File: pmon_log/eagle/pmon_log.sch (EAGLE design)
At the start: 29 parts, among them J5 microSD Socket, Q1 16Mhz, U2 LTC2943, U3 TC1015, U4 ATMEGA328TQFP32

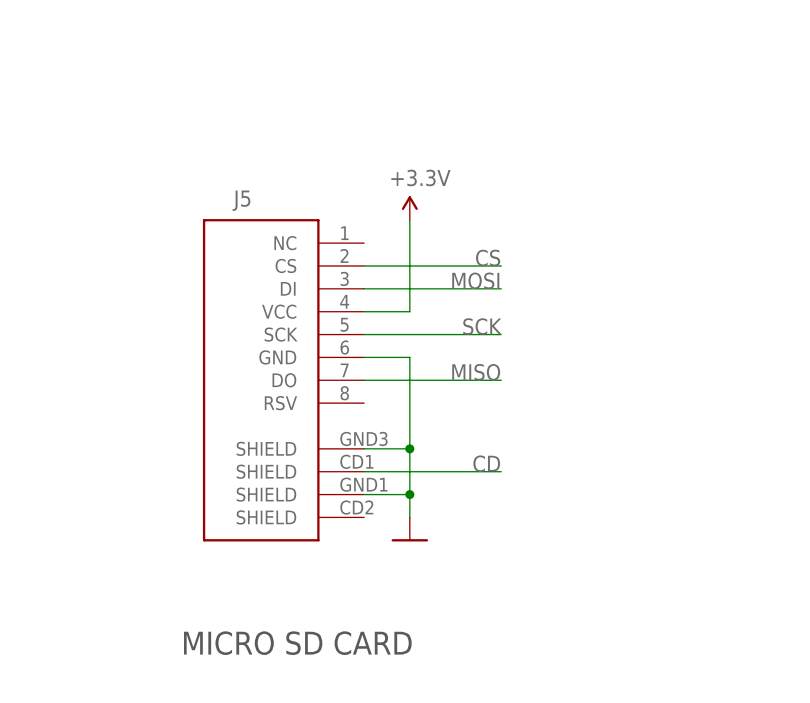
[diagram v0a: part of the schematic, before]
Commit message: Added pdf schematic.
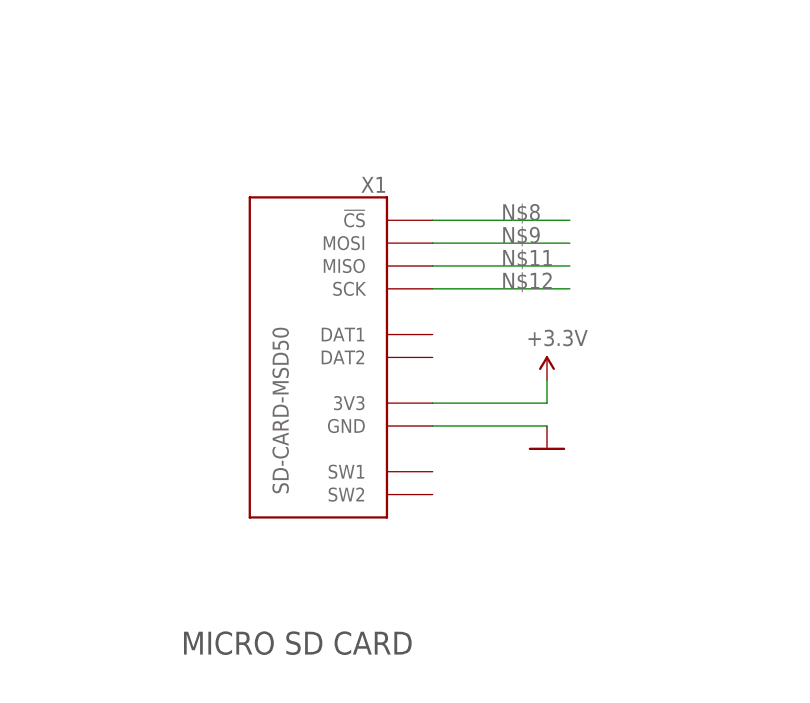
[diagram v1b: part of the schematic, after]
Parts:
- removed J5: microSD Socket, SparkFun:USD-SOCKETNEW
- added X1: SD-CARD-MSD50, pmon_log:SD-CARD-MSD50
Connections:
- new net N$11: X1.MISO
- new net N$12: X1.SCK
- new net N$8: X1.!CS
- new net N$9: X1.MOSI
- net +3.3V: now also X1.3V3; no longer J5.VCC
- net CD: no longer J5.SHIELD@2
- net CS: no longer J5.CS
- net GND: now also X1.GND; no longer J5.GND, J5.SHIELD@1, J5.SHIELD@3
- net MISO: no longer J5.DO
- net MOSI: no longer J5.DI
- net SCK: no longer J5.SCK
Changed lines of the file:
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@@
 <layer number="108" name="tplace-old" color="7" fill="1" visible="yes" active="yes"/>
 <layer number="109" name="ref-old" color="7" fill="1" visible="yes" active="yes"/>
+<layer number="110" name="fp0" color="7" fill="1" visible="yes" active="yes"/>
 <layer number="116" name="Patch_BOT" color="9" fill="4" visible="yes" active="yes"/>
 <layer number="118" name="Rect_Pads" color="7" fill="1" visible="yes" active="yes"/>
+<layer number="120" name="Descript" color="7" fill="1" visible="yes" active="yes"/>
 <layer number="121" name="_tsilk" color="7" fill="1" visible="yes" active="yes"/>
 <layer number="122" name="_bsilk" color="7" fill="1" visible="yes" active="yes"/>
+<layer number="123" name="tTestmark" color="7" fill="1" visible="yes" active="yes"/>
+<layer number="124" name="bTestmark" color="7" fill="1" visible="yes" active="yes"/>
 <layer number="125" name="_tNames" color="7" fill="1" visible="no" active="yes"/>
 <layer number="131" name="prix" color="7" fill="1" visible="yes" active="yes"/>
@@
 <part name="J1" library="pmon_log" deviceset="PINHD-1X2" device=""/>
 <part name="J2" library="pmon_log" deviceset="PINHD-1X2" device=""/>
-<part name="J5" library="SparkFun" deviceset="USD-SOCKET" device="NEW" value="microSD Socket"/>
 <part name="U$7" library="pmon_5v" deviceset="NC" device=""/>
 <part name="U$2" library="pmon_log" deviceset="+VBAT" device=""/>
@@
 <part name="D1" library="diode" deviceset="DIODE-" device="SC79_INFINEON"/>
 <part name="U$3" library="pmon_log" deviceset="+VBAT" device=""/>
-<part name="GND2" library="pmon_5v" deviceset="GND" device=""/>
-<part name="U$4" library="pmon_log" deviceset="+3.3V" device=""/>
 <part name="U$9" library="pmon_log" deviceset="+VUSB" device=""/>
 <part name="U$19" library="pmon_log" deviceset="+VUSB" device=""/>
@@
 <part name="R7" library="resistor" deviceset="R-EU_" device="R0402" value="3K3"/>
 <part name="U$6" library="pmon_5v" deviceset="NC" device=""/>
+<part name="X1" library="pmon_log" deviceset="SD-CARD" device="-MSD50"/>
+<part name="U$16" library="pmon_log" deviceset="+3.3V" device=""/>
+<part name="GND9" library="pmon_5v" deviceset="GND" device=""/>
 </parts>
 <sheets>
@@
 <attribute name="VALUE" x="44.45" y="187.96" size="1.778" layer="96"/>
 </instance>
-<instance part="J5" gate="G$1" x="17.78" y="63.5" smashed="yes" rot="MR0">
-<attribute name="NAME" x="12.954" y="80.264" size="1.778" layer="95" rot="MR0"/>
-</instance>
 <instance part="U$7" gate="G$1" x="238.76" y="172.72" rot="R180"/>
 <instance part="U$2" gate="G$1" x="7.62" y="213.36" rot="R270"/>
@@
 <instance part="U$3" gate="G$1" x="91.44" y="215.9" smashed="yes">
 <attribute name="VALUE" x="89.408" y="213.868" size="1.778" layer="96" rot="R90"/>
-</instance>
-<instance part="GND2" gate="1" x="30.48" y="43.18"/>
-<instance part="U$4" gate="G$1" x="30.48" y="78.74" smashed="yes">
-<attribute name="VALUE" x="28.194" y="82.55" size="1.778" layer="96"/>
 </instance>
 <instance part="U$9" gate="G$1" x="121.92" y="121.92" smashed="yes" rot="R270">
@@
 </instance>
 <instance part="U$6" gate="G$1" x="238.76" y="180.34" rot="R180"/>
+<instance part="X1" gate="&gt;NAME" x="20.32" y="63.5" rot="MR0"/>
+<instance part="U$16" gate="G$1" x="45.72" y="60.96" smashed="yes">
+<attribute name="VALUE" x="43.434" y="64.77" size="1.778" layer="96"/>
+</instance>
+<instance part="GND9" gate="1" x="45.72" y="53.34"/>
 </instances>
 <busses>
@@
 </segment>
 <segment>
-<wire x1="25.4" y1="63.5" x2="30.48" y2="63.5" width="0.1524" layer="91"/>
-<wire x1="30.48" y1="63.5" x2="30.48" y2="53.34" width="0.1524" layer="91"/>
-<wire x1="30.48" y1="53.34" x2="30.48" y2="48.26" width="0.1524" layer="91"/>
-<wire x1="30.48" y1="48.26" x2="30.48" y2="45.72" width="0.1524" layer="91"/>
-<wire x1="25.4" y1="53.34" x2="30.48" y2="53.34" width="0.1524" layer="91"/>
-<wire x1="25.4" y1="48.26" x2="30.48" y2="48.26" width="0.1524" layer="91"/>
-<junction x="30.48" y="53.34"/>
-<junction x="30.48" y="48.26"/>
-<pinref part="J5" gate="G$1" pin="GND"/>
-<pinref part="J5" gate="G$1" pin="SHIELD@1"/>
-<pinref part="J5" gate="G$1" pin="SHIELD@3"/>
-<pinref part="GND2" gate="1" pin="GND"/>
-</segment>
-<segment>
 <pinref part="LED1" gate="G$1" pin="C"/>
 <pinref part="GND6" gate="1" pin="GND"/>
@@
 <pinref part="GND7" gate="1" pin="GND"/>
 <wire x1="114.3" y1="55.88" x2="114.3" y2="58.42" width="0.1524" layer="91"/>
+</segment>
+<segment>
+<pinref part="X1" gate="&gt;NAME" pin="GND"/>
+<wire x1="33.02" y1="55.88" x2="45.72" y2="55.88" width="0.1524" layer="91"/>
+<pinref part="GND9" gate="1" pin="GND"/>
 </segment>
 </net>
@@
 <pinref part="U4" gate="G$1" pin="PB5(SCK)"/>
 </segment>
-<segment>
-<wire x1="25.4" y1="66.04" x2="40.64" y2="66.04" width="0.1524" layer="91"/>
-<label x="40.64" y="66.04" size="1.778" layer="95" rot="MR0"/>
-<pinref part="J5" gate="G$1" pin="SCK"/>
-</segment>
 </net>
 <net name="SER_RX" class="0">
@@
 <label x="226.06" y="119.38" size="1.778" layer="95"/>
 <pinref part="J3" gate="A" pin="MOSI"/>
-</segment>
-<segment>
-<wire x1="25.4" y1="71.12" x2="40.64" y2="71.12" width="0.1524" layer="91"/>
-<label x="40.64" y="71.12" size="1.778" layer="95" rot="MR0"/>
-<pinref part="J5" gate="G$1" pin="DI"/>
 </segment>
 </net>
@@
 <label x="190.5" y="121.92" size="1.778" layer="95"/>
 <pinref part="J3" gate="A" pin="MISO"/>
-</segment>
-<segment>
-<wire x1="25.4" y1="60.96" x2="40.64" y2="60.96" width="0.1524" layer="91"/>
-<label x="40.64" y="60.96" size="1.778" layer="95" rot="MR0"/>
-<pinref part="J5" gate="G$1" pin="DO"/>
 </segment>
 </net>
@@
 <net name="CS" class="0">
 <segment>
-<wire x1="25.4" y1="73.66" x2="40.64" y2="73.66" width="0.1524" layer="91"/>
-<label x="40.64" y="73.66" size="1.778" layer="95" rot="MR0"/>
-<pinref part="J5" gate="G$1" pin="CS"/>
-</segment>
-<segment>
 <pinref part="U4" gate="G$1" pin="PB2(SS/OC1B)"/>
 <wire x1="238.76" y1="162.56" x2="259.08" y2="162.56" width="0.1524" layer="91"/>
@@
 </net>
 <net name="CD" class="0">
-<segment>
-<wire x1="25.4" y1="50.8" x2="40.64" y2="50.8" width="0.1524" layer="91"/>
-<label x="40.64" y="50.8" size="1.778" layer="95" rot="MR0"/>
-<pinref part="J5" gate="G$1" pin="SHIELD@2"/>
-</segment>
 <segment>
 <pinref part="U4" gate="G$1" pin="PC2(ADC2)"/>
@@
 </segment>
 </net>
-<net name="+3.3V" class="0">
-<segment>
-<wire x1="25.4" y1="68.58" x2="30.48" y2="68.58" width="0.1524" layer="91"/>
-<wire x1="30.48" y1="68.58" x2="30.48" y2="78.74" width="0.1524" layer="91"/>
-<pinref part="J5" gate="G$1" pin="VCC"/>
-<pinref part="U$4" gate="G$1" pin="+3.3V"/>
-</segment>
-</net>
 <net name="+USB" class="0">
 <segment>
@@
 </segment>
 </net>
+<net name="N$8" class="0">
+<segment>
+<pinref part="X1" gate="&gt;NAME" pin="!CS"/>
+<wire x1="33.02" y1="78.74" x2="48.26" y2="78.74" width="0.1524" layer="91"/>
+<label x="40.64" y="78.74" size="1.778" layer="95"/>
+</segment>
+</net>
+<net name="N$9" class="0">
+<segment>
+<pinref part="X1" gate="&gt;NAME" pin="MOSI"/>
+<wire x1="33.02" y1="76.2" x2="48.26" y2="76.2" width="0.1524" layer="91"/>
+<label x="40.64" y="76.2" size="1.778" layer="95"/>
+</segment>
+</net>
+<net name="N$11" class="0">
+<segment>
+<pinref part="X1" gate="&gt;NAME" pin="MISO"/>
+<wire x1="33.02" y1="73.66" x2="48.26" y2="73.66" width="0.1524" layer="91"/>
+<label x="40.64" y="73.66" size="1.778" layer="95"/>
+</segment>
+</net>
+<net name="N$12" class="0">
+<segment>
+<pinref part="X1" gate="&gt;NAME" pin="SCK"/>
+<wire x1="33.02" y1="71.12" x2="48.26" y2="71.12" width="0.1524" layer="91"/>
+<label x="40.64" y="71.12" size="1.778" layer="95"/>
+</segment>
+</net>
+<net name="+3.3V" class="0">
+<segment>
+<pinref part="X1" gate="&gt;NAME" pin="3V3"/>
+<wire x1="33.02" y1="58.42" x2="45.72" y2="58.42" width="0.1524" layer="91"/>
+<wire x1="45.72" y1="58.42" x2="45.72" y2="60.96" width="0.1524" layer="91"/>
+<pinref part="U$16" gate="G$1" pin="+3.3V"/>
+</segment>
+</net>
